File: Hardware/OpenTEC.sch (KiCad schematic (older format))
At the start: 72 parts, among them J1 USB_B_Micro, J10 TEMP3, J11 TEC_A, J12 TEC_B, J13 XH2.54, J14 XH2.54, J15 XH2.54, J16 XH2.54, J17 XH2.54, J18 XH2.54, J19 XH2.54, J2 4P Screw Terminal, J20 XH2.54, J21 XH2.54, J22 XH2.54, J23 XH2.54, J24 XH2.54, J25 XH2.54, J26 XH2.54, J27 XH2.54, J28 XH2.54, J3 10P JTAG/SWD, J4 LCD, J5 I2C, J6 BOOT_SEL, J7 TEMP0, J8 TEMP1, J9 TEMP2, U1 AMS1117-5.0, U10 EL357N, U11 STM32F103C8T6, U2 AMS1117-3.3, U3 DMC3021LK4, U4 DMC3021LK4, U5 EL357N, U6 EL357N, U7 DMC3021LK4, U8 DMC3021LK4, U9 EL357N, Y1 16MHz

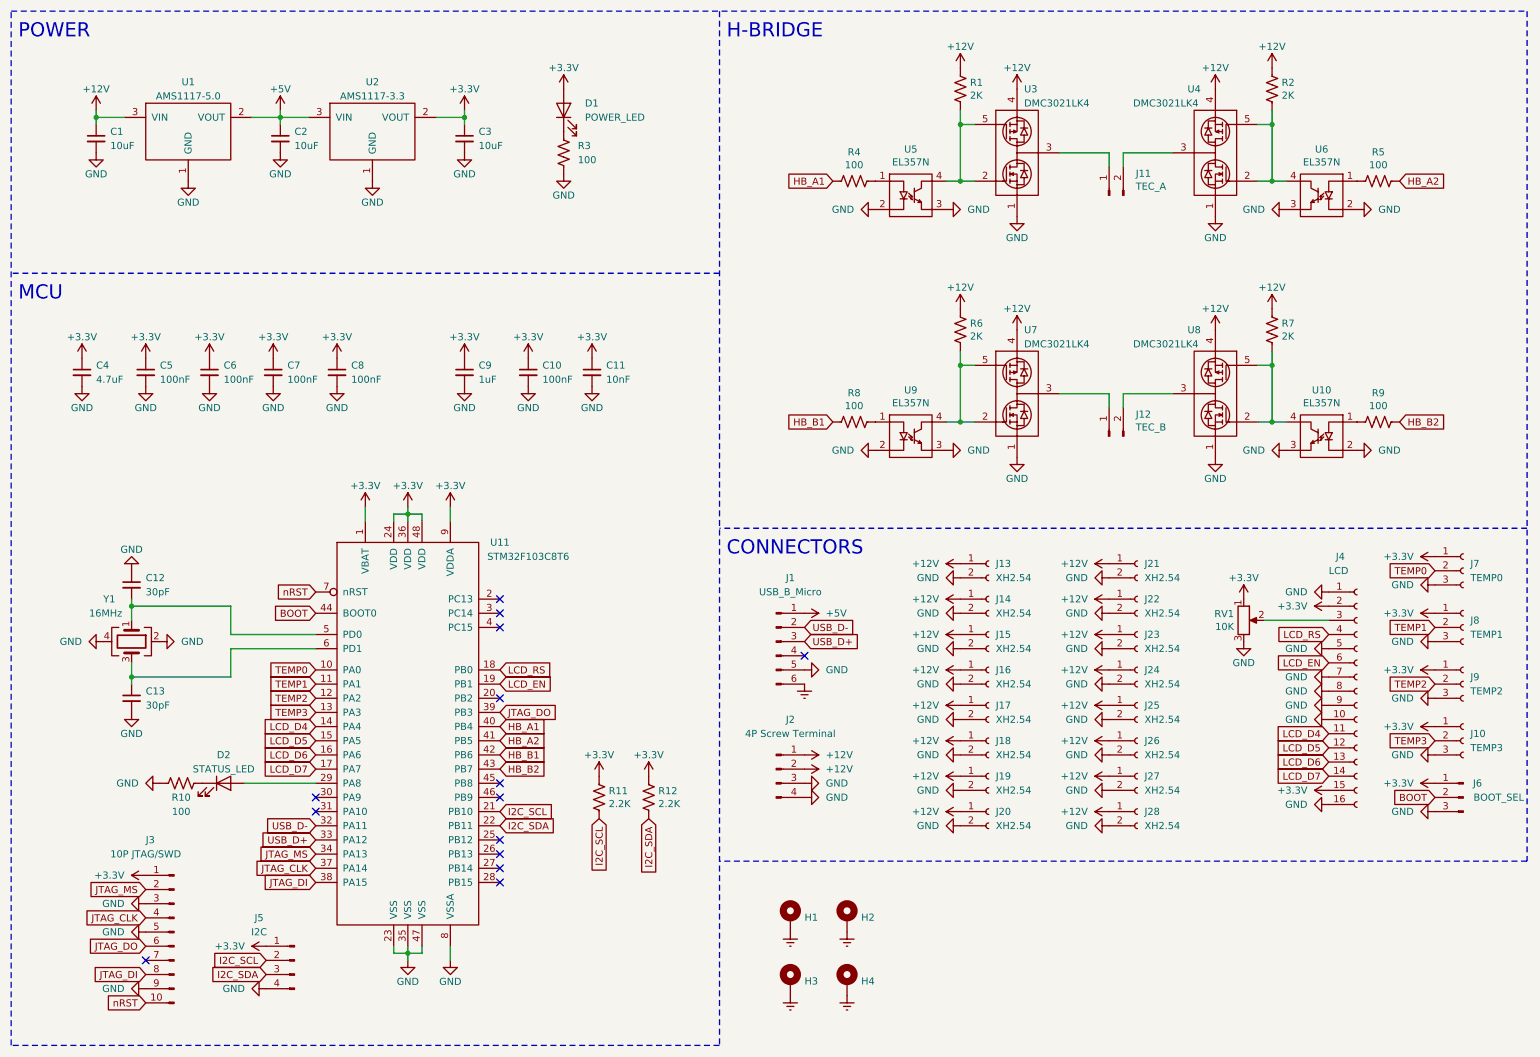
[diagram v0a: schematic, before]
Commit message: Change H-bridge design
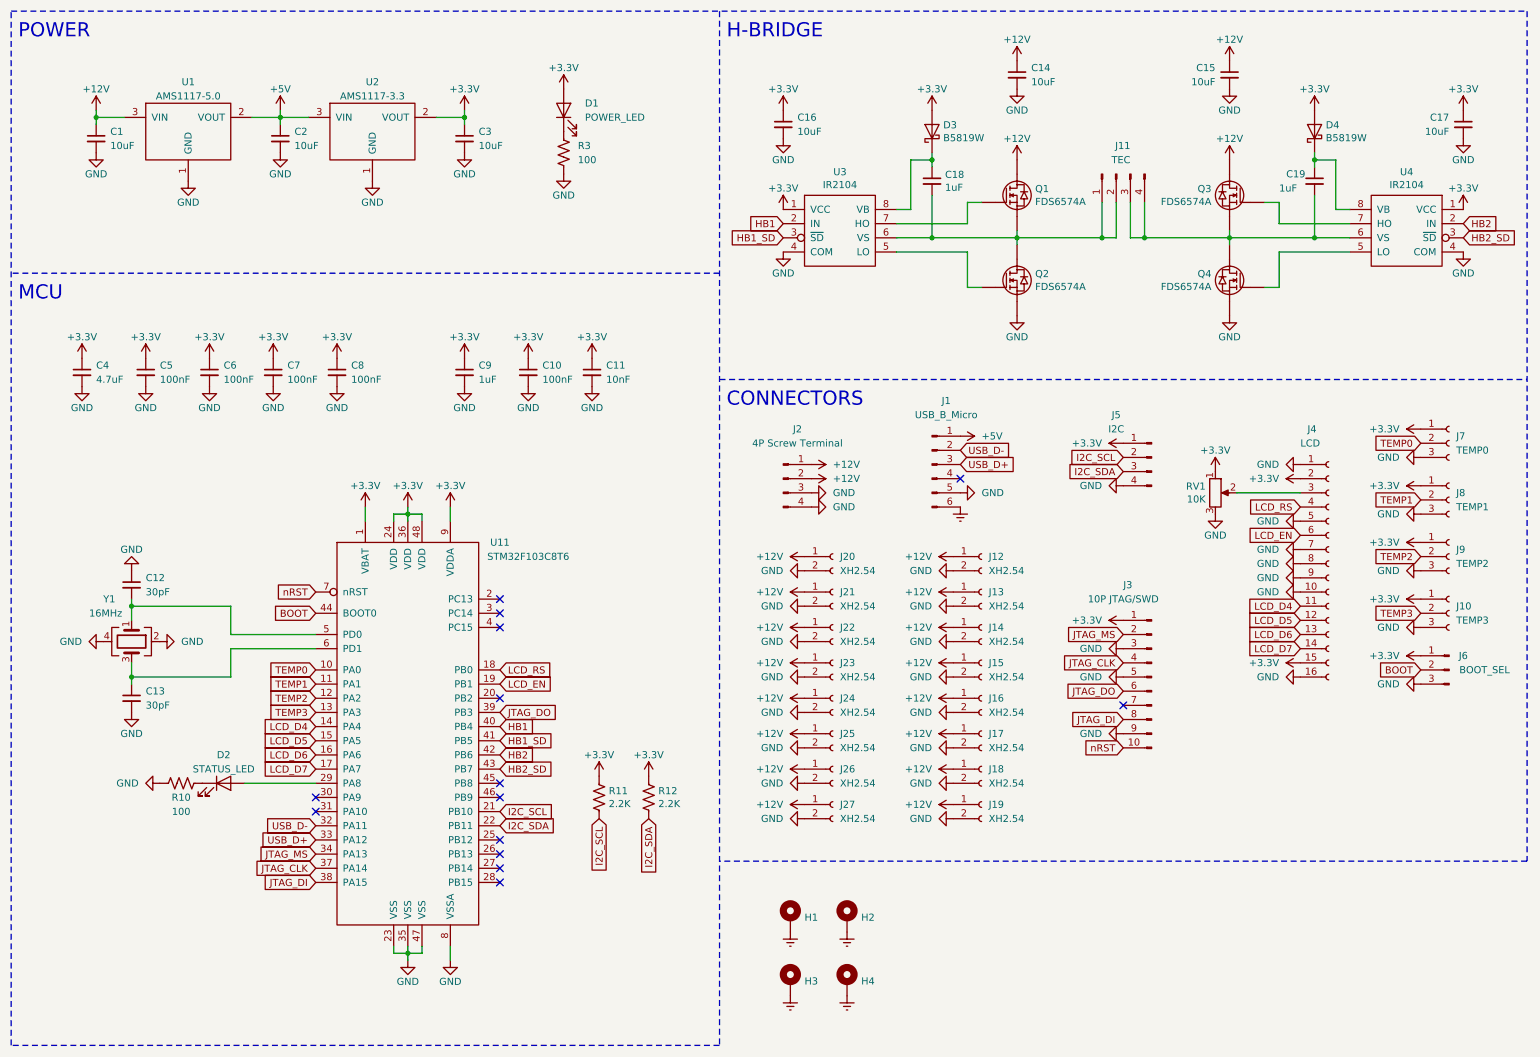
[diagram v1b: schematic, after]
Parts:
- removed J11: TEC_A, TerminalBlock:TerminalBlock_bornier-2_P5.08mm, symbol Connector:Conn_01x02_Male
- removed J12: TEC_B, TerminalBlock:TerminalBlock_bornier-2_P5.08mm, symbol Connector:Conn_01x02_Male
- removed R1, R2, R6, R7: 2K, Resistor_SMD:R_1206_3216Metric, symbol Device:R_US
- removed R4, R5, R8, R9: 100, Resistor_SMD:R_0402_1005Metric, symbol Device:R_US
- removed U10, U5, U6, U9: EL357N, Package_SO:SOP-4_3.8x4.1mm_P2.54mm, symbol OpenTEC:EL357N
- removed U3, U4, U7, U8: DMC3021LK4, Package_TO_SOT_SMD:TO-252-4, symbol OpenTEC:DMC3021LK4
- added C14, C15, C16, C17: 10uF, Capacitor_SMD:C_0805_2012Metric, symbol Device:C_Small
- added C18, C19: 1uF, Capacitor_SMD:C_0805_2012Metric, symbol Device:C_Small
- added D3, D4: B5819W, Diode_SMD:D_SOD-123, symbol Device:D_Schottky
- added J11: TEC, TerminalBlock:TerminalBlock_bornier-4_P5.08mm, symbol Connector:Conn_01x04_Male
- added Q1, Q2, Q3, Q4: FDS6574A, Package_SO:SOIC-8_3.9x4.9mm_P1.27mm, symbol OpenTEC:FDS6574A
- added U3, U4: IR2104, Package_SO:SOIC-8_3.9x4.9mm_P1.27mm, symbol OpenTEC:IR2104
- renumbered J28 to J12
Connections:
- net +12V: now also C14.1, C15.1, Q1.5, Q1.6, Q1.7, Q1.8, Q3.5, Q3.6, Q3.7, Q3.8
- net +3V3: now also C16.1, C17.1, D3.2 (A), D4.2 (A), U3.1 (VCC), U4.1 (VCC)
- net GND: now also C14.2, C15.2, C16.2, C17.2, Q2.1, Q2.2, Q2.3, Q4.1, Q4.2, Q4.3, U3.4 (COM), U4.4 (COM)
- net HB_A1 renamed HB1
- net HB1: now also U3.2 (IN)
- net HB_A2 renamed HB1_SD
- net HB1_SD: now also U3.3 (~SD)
- net HB_B1 renamed HB2
- net HB2: now also U4.2 (IN)
- net HB_B2 renamed HB2_SD
- net HB2_SD: now also U4.3 (~SD)
- new net: C18.2, J11.1 (Pin_1), J11.2 (Pin_2), Q1.1, Q1.2, Q1.3, Q2.5, Q2.6, Q2.7, Q2.8, U3.6 (VS)
- new net: Q1.4, U3.7 (HO)
- new net: Q2.4, U3.5 (LO)
- new net: C19.2, J11.3 (Pin_3), J11.4 (Pin_4), Q3.1, Q3.2, Q3.3, Q4.5, Q4.6, Q4.7, Q4.8, U4.6 (VS)
- new net: Q3.4, U4.7 (HO)
- new net: Q4.4, U4.5 (LO)
- new net: C18.1, D3.1 (K), U3.8 (VB)
- new net: C19.1, D4.1 (K), U4.8 (VB)
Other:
- moved on the sheet: J1, J10, J12, J13, J14, J15, J16, J17, J18, J19, J2, J20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
